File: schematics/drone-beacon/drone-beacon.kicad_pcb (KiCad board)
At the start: 2 copper layers, 23.3 x 29.9 mm, 13 parts, among them J1 ESP32 Flashing connector, J2 Power Input, SW1 Model selection, U1 ESP32-WROOM-32U, U2 AMS1117-3.3, U3 L80-R

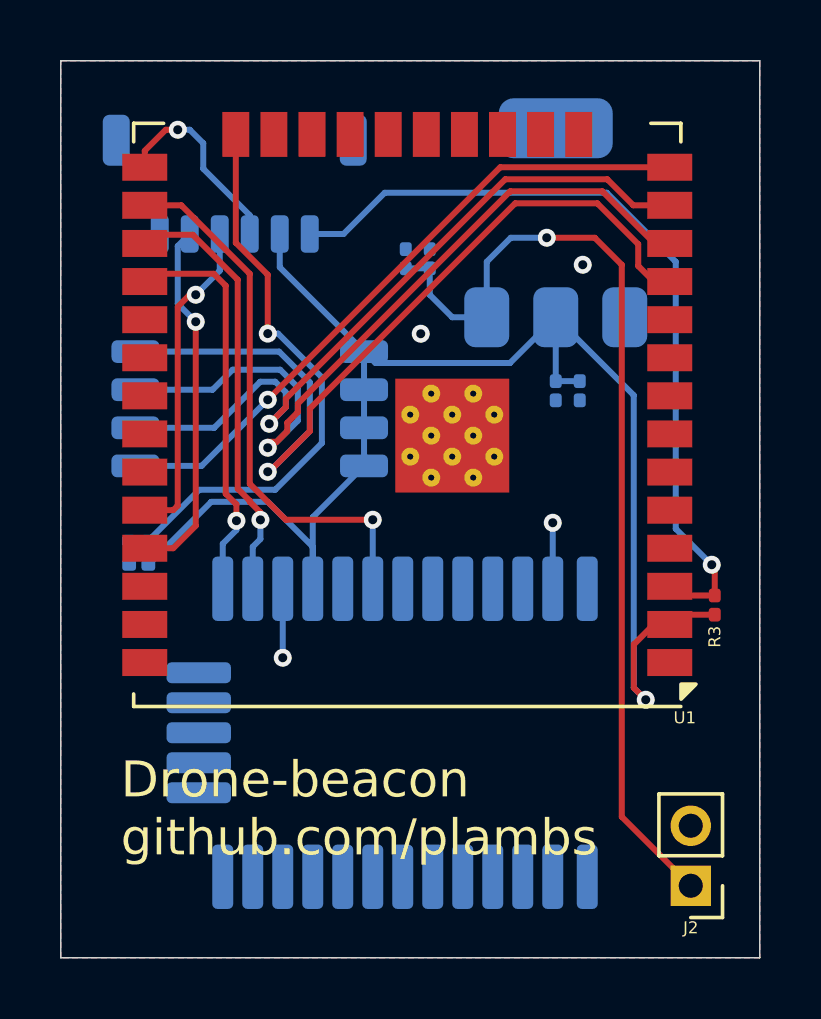
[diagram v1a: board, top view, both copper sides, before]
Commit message: Update schematics
Signed-off-by: LAMBS Pierre-Antoine <pierreantoine.lambs@gmail.com>
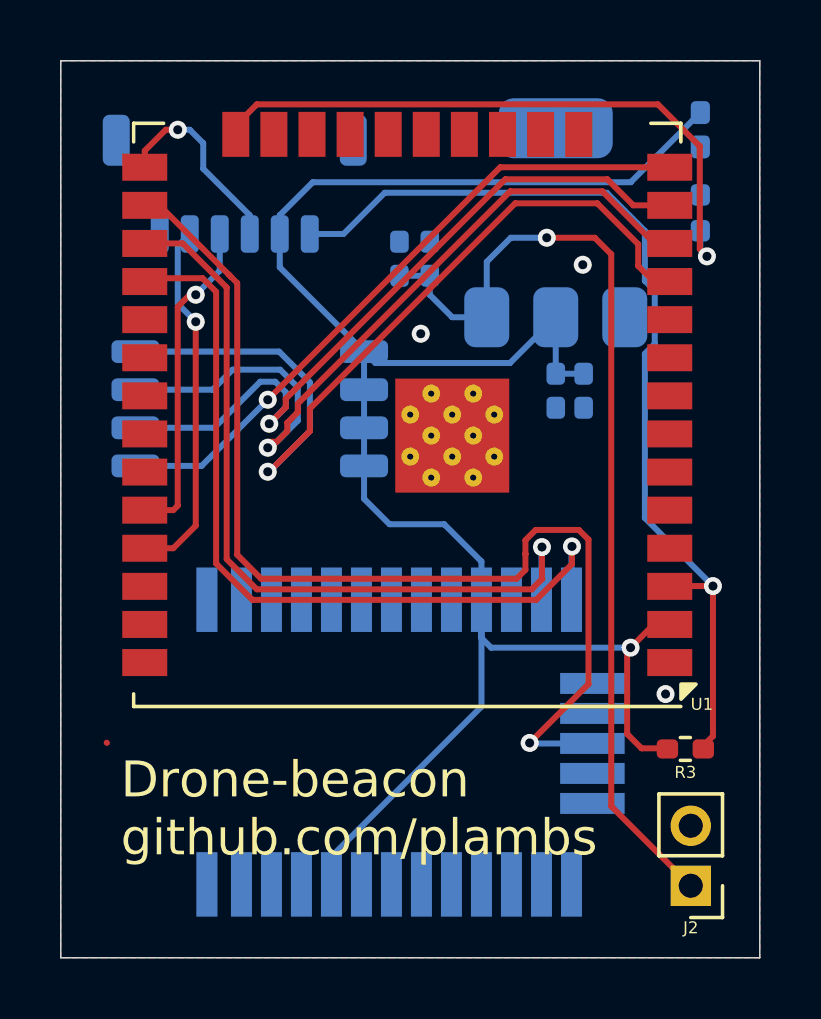
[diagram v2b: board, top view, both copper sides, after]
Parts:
- C1, C2, C3, C4: footprint Capacitor_SMD:C_0201_0603Metric -> Capacitor_SMD:C_0402_1005Metric_Pad0.74x0.62mm_HandSolder
- D1: footprint LED_SMD:LED_0201_0603Metric -> LED_SMD:LED_0402_1005Metric_Pad0.77x0.64mm_HandSolder
- R1, R3: footprint Resistor_SMD:R_0201_0603Metric -> Resistor_SMD:R_0402_1005Metric_Pad0.72x0.64mm_HandSolder
- U3: value L80-R -> L96; footprint RF_GPS:Quectel_L96 -> QUECTEL_L96:L96
- moved D1 23.7 mm to (200.8, 51.9), turned to 90 degrees
- moved R1 21.7 mm to (200.8, 54.7), turned to 90 degrees
- moved R3 4.89 mm to (200.3, 72.5), turned to 0 degrees
- moved U3 0.42 mm to (190.8, 72.3)
- moved C2 0.21 mm to (190.8, 56.2)
- moved C3 0.13 mm to (196.9, 60.6)
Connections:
- U3 pad 1: /GPS_RX -> unconnected-(U3-NC1-Pad1)
- U3 pad 10: unconnected-(U3-~{RESET}-Pad10) -> GND
- U3 pad 11: unconnected-(U3-RESERVED-Pad11) -> GND
- U3 pad 13: (no net) -> GND
- U3 pad 14: (no net) -> GND
- U3 pad 15: (no net) -> GND
- U3 pad 16: (no net) -> unconnected-(U3-RF_OUT-Pad16)
- U3 pad 17: (no net) -> unconnected-(U3-RF_IN-Pad17)
- U3 pad 18: (no net) -> GND
- U3 pad 19: (no net) -> GND
- U3 pad 2: /GPS_TX -> unconnected-(U3-3D_FIX-Pad2)
- U3 pad 20: (no net) -> unconnected-(U3-JAM_DET-Pad20)
- U3 pad 21: (no net) -> GND
- U3 pad 22: (no net) -> GND
- U3 pad 23: (no net) -> +3.3V
- U3 pad 24: (no net) -> unconnected-(U3-GEO_FENCE-Pad24)
- U3 pad 25: (no net) -> /GPS_TX
- U3 pad 26: (no net) -> /GPS_RX
- U3 pad 27: (no net) -> GND
- U3 pad 28: (no net) -> unconnected-(U3-FORCE_ON-Pad28)
- U3 pad 29: (no net) -> /GPS_PPS
- U3 pad 3: GND -> unconnected-(U3-I2C_SDA-Pad3)
- U3 pad 30: (no net) -> unconnected-(U3-ANTON-Pad30)
- U3 pad 31: (no net) -> GND
- U3 pad 4: +3.3V -> GND
- U3 pad 5: unconnected-(U3-V_BCKP-Pad5) -> GND
- U3 pad 6: /GPS_PPS -> unconnected-(U3-I2C_SCL-Pad6)
- U3 pad 9: unconnected-(U3-NC-Pad9) -> +3.3V
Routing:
- net /GPS_PPS: track 18.3 -> 36.3 mm
- net +3.3V: track 51.3 -> 66.1 mm
- net /GPS_RX: track 13.4 -> 26.9 mm
- net /GPS_TX: track 14.6 -> 26.3 mm
- net /ESP32_EN: track 27.0 -> 32.3 mm
- net GND: track 4.50 -> 0.01 mm, vias 4 -> 3
- net /STATUS_LED: track 18.8 -> 21.4 mm
- net Net-(D1-K): track 0.80 -> 0.00 mm

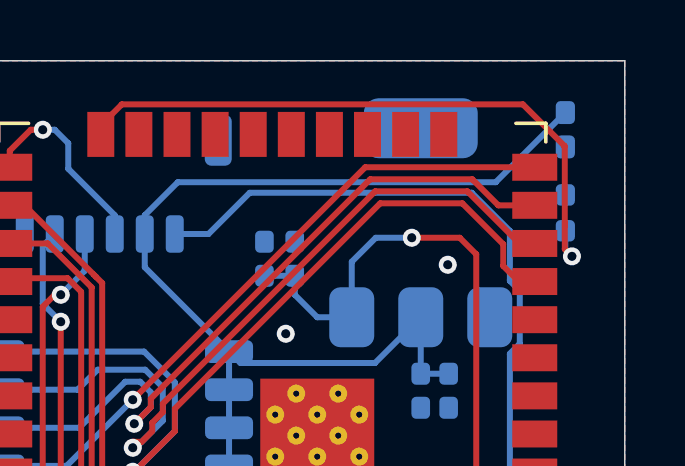
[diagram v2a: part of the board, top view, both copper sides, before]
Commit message: Update schematics (WIP)
Signed-off-by: LAMBS Pierre-Antoine <pierreantoine.lambs@gmail.com>
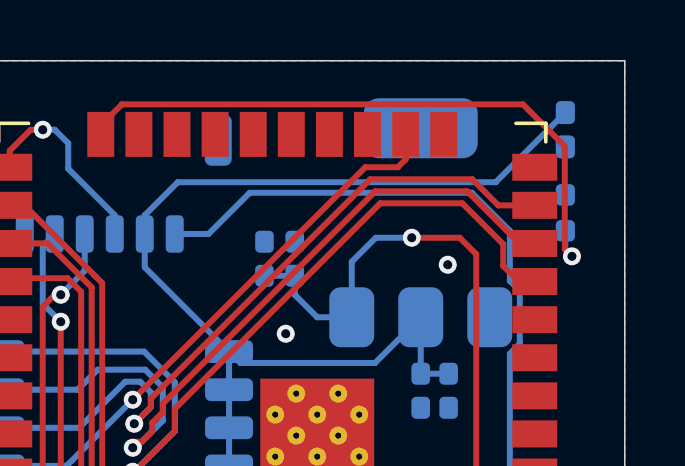
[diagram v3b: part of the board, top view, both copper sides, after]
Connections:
- U1 pad 14: /DIP1 -> unconnected-(U1-IO12-Pad14)
- U1 pad 16: unconnected-(U1-IO13-Pad16) -> /DIP1
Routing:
- net /DIP1: track 21.9 -> 18.6 mm
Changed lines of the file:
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@@
 	(net 21 "unconnected-(U1-SHD{slash}SD2-Pad17)")
 	(net 22 "unconnected-(U1-IO33-Pad9)")
-	(net 23 "unconnected-(U1-IO13-Pad16)")
+	(net 23 "unconnected-(U1-IO12-Pad14)")
 	(net 24 "unconnected-(U1-IO18-Pad30)")
 	(net 25 "unconnected-(U1-IO5-Pad29)")
@@
 			(size 1.5 0.9)
 			(layers "F.Cu" "F.Mask" "F.Paste")
-			(net 10 "/DIP1")
+			(net 23 "unconnected-(U1-IO12-Pad14)")
 			(pinfunction "IO12")
-			(pintype "bidirectional")
+			(pintype "bidirectional+no_connect")
 		)
 		(pad "15" smd rect
@@
 			(size 1.5 0.9)
 			(layers "F.Cu" "F.Mask" "F.Paste")
-			(net 23 "unconnected-(U1-IO13-Pad16)")
+			(net 10 "/DIP1")
 			(pinfunction "IO13")
-			(pintype "bidirectional+no_connect")
+			(pintype "bidirectional")
 		)
 		(pad "17" smd rect
@@
 	)
 	(segment
-		(start 199.8 53.15)
-		(end 194.15 53.15)
+		(start 194.15 53.15)
+		(end 195.236 53.15)
+		(width 0.2)
+		(layer "F.Cu")
+		(net 10)
+	)
+	(segment
+		(start 195.236 53.15)
+		(end 195.495 52.891)
 		(width 0.2)
 		(layer "F.Cu")
@@
 		(width 0.2)
 		(layer "F.Cu")
+		(net 10)
+	)
+	(segment
+		(start 195.495 52.891)
+		(end 195.495 52.055)
+		(width 0.2)
+		(layer "F.Cu")

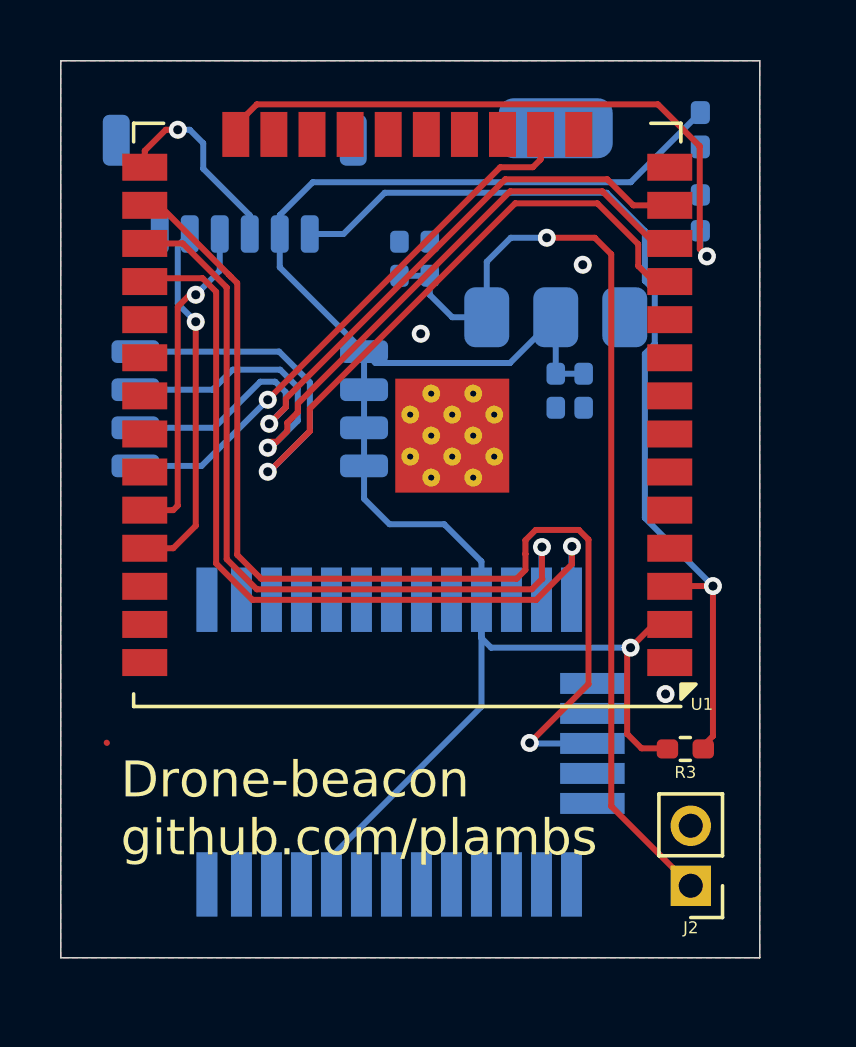
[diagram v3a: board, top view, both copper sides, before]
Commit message: Update schematics
Signed-off-by: LAMBS Pierre-Antoine <pierreantoine.lambs@gmail.com>
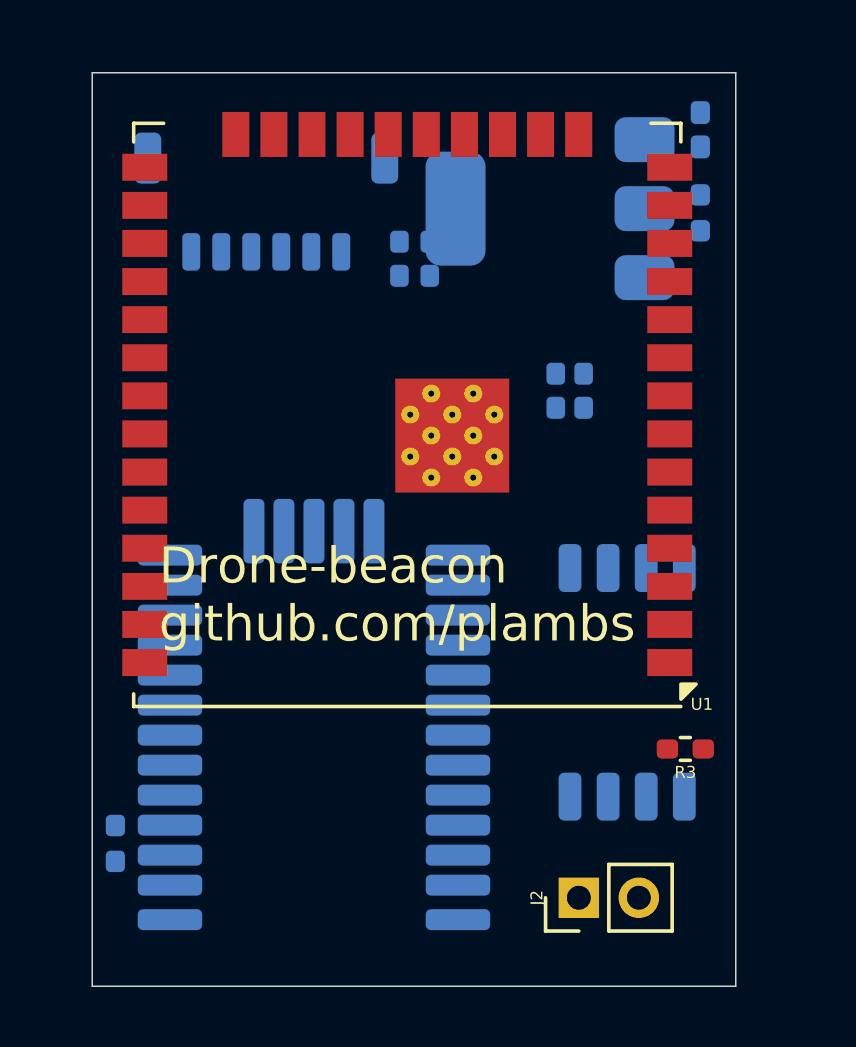
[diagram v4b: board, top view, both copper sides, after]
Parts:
- added R2: 0, Resistor_SMD:R_0402_1005Metric_Pad0.72x0.64mm_HandSolder, B.Cu at (181.3, 75.7)
- U3: footprint QUECTEL_L96:L96 -> RF_GPS:Quectel_L96
- moved SW1 15.5 mm to (198.4, 70.3), turned to 90 degrees
- moved J2 3.75 mm to (196.8, 77.5), turned to 90 degrees
- moved U3 2.87 mm to (187.9, 72.3), turned to 180 degrees
- moved J1 1.21 mm to (186.3, 54.3)
- moved U2 0.51 mm to (195.8, 54.5), turned to 180 degrees
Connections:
- C1 pad 1: Net-(J2-Pin_1) -> /VIN
- C2 pad 1: Net-(J2-Pin_1) -> /VIN
- J2 pad 1: Net-(J2-Pin_1) -> GND
- J2 pad 2: GND -> /VIN
- U2 pad 3: Net-(J2-Pin_1) -> /VIN
- U3 pad 16: unconnected-(U3-RF_OUT-Pad16) -> /RF_OUT
- U3 pad 17: unconnected-(U3-RF_IN-Pad17) -> /RF_IN
- U3 pad 8: unconnected-(U3-V_BCKP-Pad8) -> +3.3V
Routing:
- net +3.3V: track 66.1 -> 0.00 mm, vias 1 -> 0
- net /GPS_PPS: track 36.3 -> 0.00 mm, vias 1 -> 0
- net Net-(J2-Pin_1): track 32.6 -> 0.00 mm, vias 1 -> 0
- net /ESP32_EN: track 32.3 -> 0.00 mm, vias 1 -> 0
- net /DIP4: track 28.9 -> 0.00 mm, vias 1 -> 0
- net /GPS_RX: track 26.9 -> 0.00 mm, vias 1 -> 0
- net /DIP3: track 26.5 -> 0.00 mm, vias 1 -> 0
- net /GPS_TX: track 26.3 -> 0.00 mm, vias 1 -> 0
- net /DIP2: track 24.3 -> 0.00 mm, vias 1 -> 0
- net /STATUS_LED: track 21.4 -> 0.00 mm, vias 1 -> 0
- net /DIP1: track 18.6 -> 0.00 mm, vias 1 -> 0
- net /ESP32_TX: track 12.1 -> 0.00 mm, vias 1 -> 0
- net /ESP32_RX: track 10.9 -> 0.00 mm, vias 1 -> 0
- net /ESP32_BOOT: track 6.64 -> 0.00 mm, vias 1 -> 0
- net GND: track 0.01 -> 0.00 mm, vias 3 -> 0
- removed copper zone on B.Cu, net GND
- removed copper zone on F.Cu, net GND
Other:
- board size 23.3 x 29.9 mm -> 21.4 x 30.5 mm

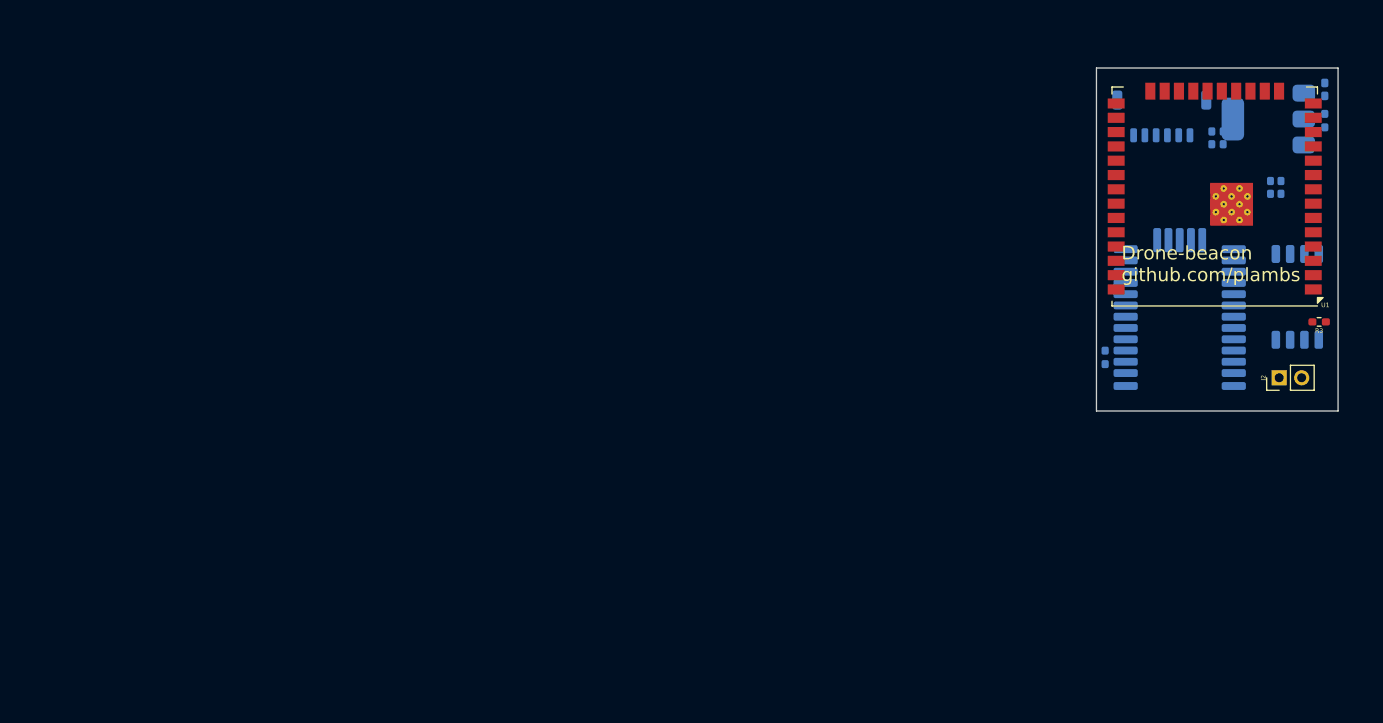
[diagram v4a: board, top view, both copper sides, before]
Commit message: Update schematics v1
Signed-off-by: LAMBS Pierre-Antoine <pierreantoine.lambs@gmail.com>
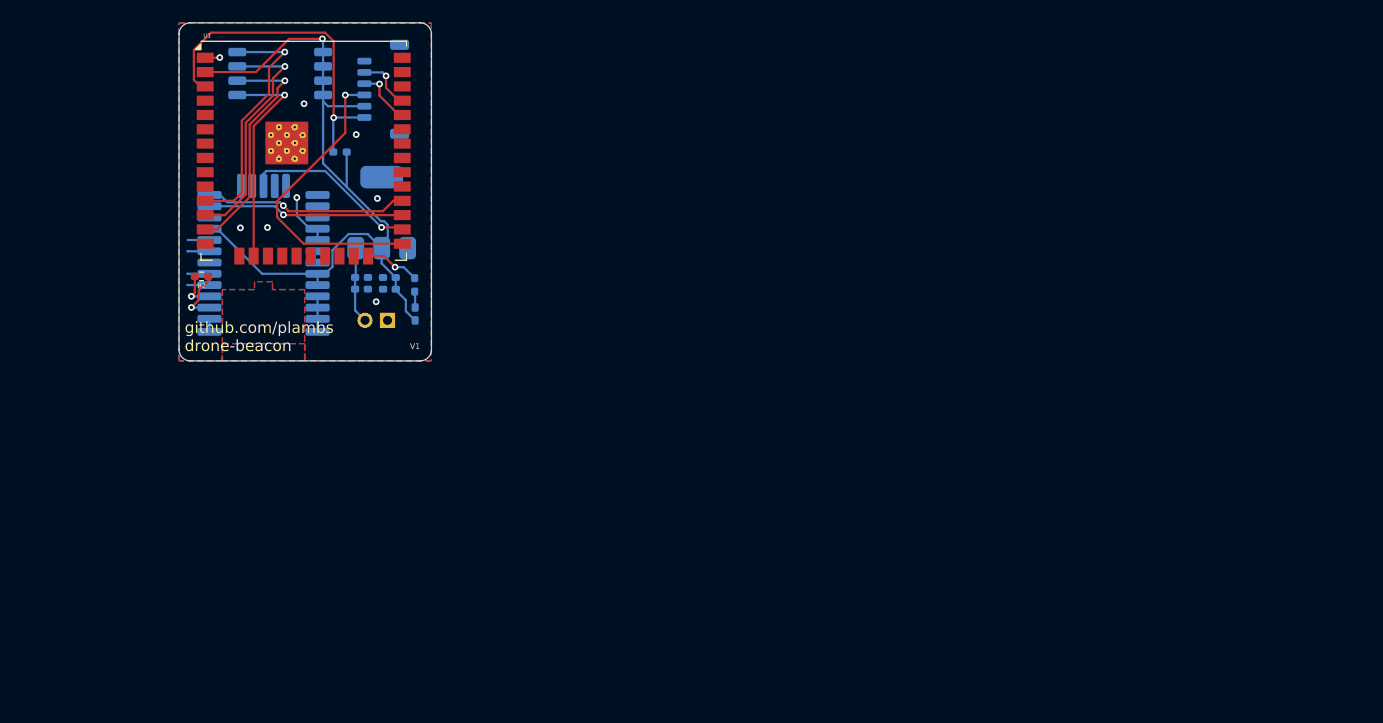
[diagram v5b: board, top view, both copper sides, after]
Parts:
- J2, R3: moved to B.Cu
- R2: moved to F.Cu
- moved SW1 92.5 mm to (108.1, 50.5), turned to 0 degrees
- moved R3 88.2 mm to (113.4, 57.5), turned to 180 degrees
- moved D1 83.2 mm to (120.1, 71.8), turned to -90 degrees
- moved R1 82.1 mm to (120.0, 69.2), turned to -90 degrees
- moved U3 81.5 mm to (106.6, 67.5)
- moved U1 81.0 mm to (110.2, 57.3), turned to 0 degrees
- moved R2 80.5 mm to (101.1, 68.5), turned to 0 degrees
- moved C3 79.7 mm to (117.8, 69.6), turned to 180 degrees
- moved J2 79.3 mm to (117.6, 72.4)
- moved U2 79.2 mm to (117.1, 62.8), turned to 90 degrees
- moved C4 78.6 mm to (117.8, 68.6), turned to 180 degrees
- moved C1 77.5 mm to (115.3, 68.6), turned to 0 degrees
- moved C2 76.7 mm to (115.3, 69.6), turned to 0 degrees
- moved J1 69.2 mm to (117.2, 51.9), turned to -90 degrees
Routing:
- net +3.3V: track 0.00 -> 68.4 mm, vias 0 -> 1
- net /ESP32_EN: track 0.00 -> 30.2 mm, vias 0 -> 1
- net /ESP32_BOOT: track 0.00 -> 27.1 mm, vias 0 -> 1
- net /DIP4: track 0.00 -> 21.8 mm, vias 0 -> 1
- net /DIP3: track 0.00 -> 21.4 mm, vias 0 -> 1
- net /DIP2: track 0.00 -> 21.0 mm, vias 0 -> 1
- net GND: track 0.00 -> 20.3 mm, vias 0 -> 8
- net /DIP1: track 0.00 -> 19.6 mm, vias 0 -> 1
- net /GPS_RX: track 0.00 -> 18.2 mm, vias 0 -> 1
- net /GPS_TX: track 0.00 -> 17.4 mm, vias 0 -> 1
- net /GPS_PPS: track 0.00 -> 15.6 mm, vias 0 -> 1
- net /VIN: track 0.00 -> 6.80 mm
- net /ESP32_RX: track 0.00 -> 5.12 mm, vias 0 -> 1
- net /ESP32_TX: track 0.00 -> 5.03 mm, vias 0 -> 1
- net /RF_OUT: track 0.00 -> 4.99 mm, vias 0 -> 1
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- added copper zone on B.Cu, net GND
- added copper zone on F.Cu, net GND
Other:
- board size 21.4 x 30.5 mm -> 22.4 x 30 mm
- board text added: "V1"
- board text added: "github.com/plambs drone-beacon"
- board text removed: "Drone-beacon github.com/plambs"
